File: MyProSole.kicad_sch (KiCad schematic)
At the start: 22 parts, among them J1 FSR3, J2 FSR2, J3 FSR3, J4 Conn_01x07_Socket_XIAO_ESP32C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, J5 i2c-bus, J6 SD_CardSocket, J7 XIAO_ESP32C3, J8 SD_CardSocketDummy

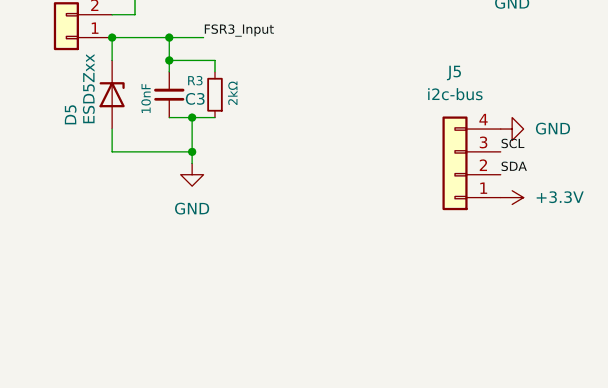
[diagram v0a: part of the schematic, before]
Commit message: Version 1.1
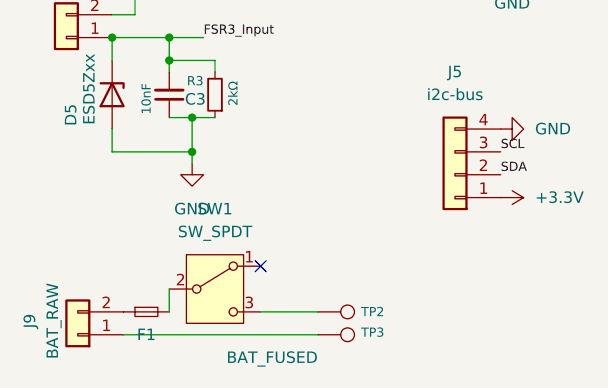
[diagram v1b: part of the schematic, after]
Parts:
- added F1: BAT_FUSED, Fuse:Fuse_1206_3216Metric_Pad1.42x1.75mm_HandSolder, symbol Device:Fuse_Small
- added J9: BAT_RAW, Connector_JST:JST_PH_B2B-PH-K_1x02_P2.00mm_Vertical, symbol Connector_Generic:Conn_01x02
- added SW1: SW_SPDT, MyProSoleLibrary:WS-SLTU THT Mini Slide Switch, symbol Switch:SW_SPDT
- added TP2, TP3: TestPoint, TestPoint:TestPoint_Pad_2.0x2.0mm, symbol Connector:TestPoint
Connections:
- new net: SW1.3 (C), TP2.1
- new net: F1.1, J9.2 (Pin_2)
- new net: F1.2, SW1.2 (B)
- new net: J9.1 (Pin_1), TP3.1
- no-connect marks 7 -> 8
